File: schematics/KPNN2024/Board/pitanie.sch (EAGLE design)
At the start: 32 parts

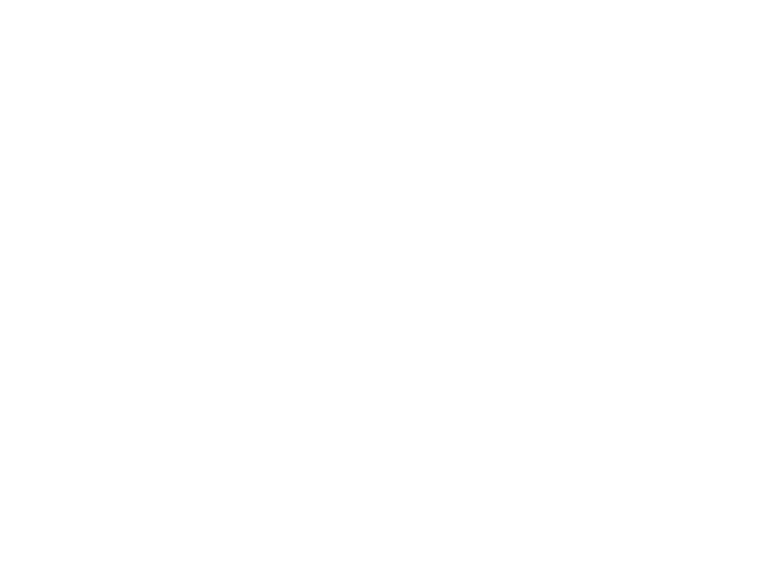
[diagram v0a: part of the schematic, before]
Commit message: я смотрел рика и морти вместо работать
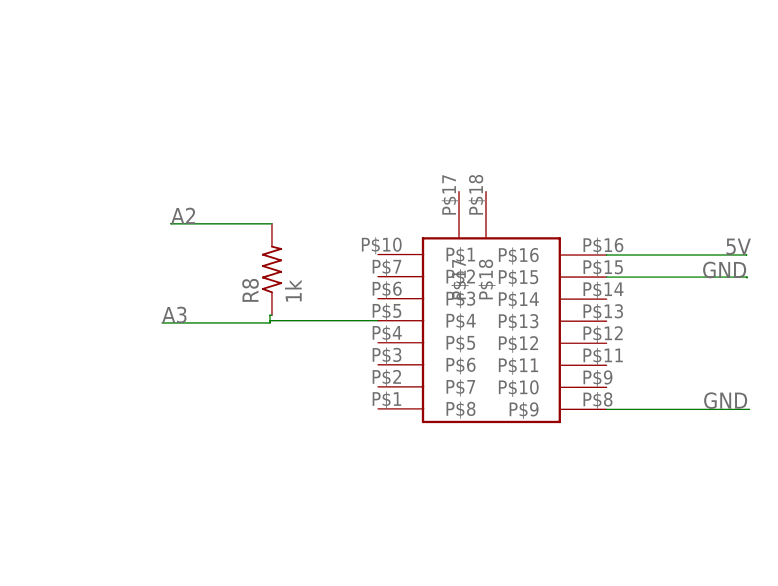
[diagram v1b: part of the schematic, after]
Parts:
- added R8: 1k, rcl:R-US_R0603
- added TMC: DRIVER_TMC2209, UNKNOWN-2024:DRIVER_TMC2209
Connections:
- new net 5V: TMC.P$16
- new net A2: R8.2
- new net A3: R8.1, TMC.P$4
- net GND: now also TMC.P$15, TMC.P$9
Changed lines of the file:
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@@
 <setting verticaltext="up"/>
 </settings>
-<grid distance="0.1" unitdist="inch" unit="inch" style="lines" multiple="1" display="no" altdistance="0.01" altunitdist="inch" altunit="inch"/>
+<grid distance="1" unitdist="mm" unit="mm" style="lines" multiple="1" display="no" altdistance="0.05" altunitdist="mm" altunit="mm"/>
 <layers>
 <layer number="1" name="Top" color="4" fill="1" visible="no" active="no"/>
@@
 <part name="LIS" library="CanCubeSat" deviceset="LIS3MDL-GY" device=""/>
 <part name="R7" library="rcl" library_urn="urn:adsk.eagle:library:334" deviceset="R-US_" device="R0603" package3d_urn="urn:adsk.eagle:package:23555/3" value="2k"/>
+<part name="TMC" library="UNKNOWN-2024" deviceset="DRIVER_TMC2209" device=""/>
+<part name="R8" library="rcl" library_urn="urn:adsk.eagle:library:334" deviceset="R-US_" device="R0603" package3d_urn="urn:adsk.eagle:package:23555/3" value="1k"/>
 </parts>
 <sheets>
@@
 <attribute name="NAME" x="117.8814" y="85.09" size="1.778" layer="95" rot="R90"/>
 <attribute name="VALUE" x="122.682" y="85.09" size="1.778" layer="96" rot="R90"/>
+</instance>
+<instance part="TMC" gate="G$1" x="362" y="78" smashed="yes"/>
+<instance part="R8" gate="G$1" x="345.22" y="94.94" smashed="yes" rot="R90">
+<attribute name="NAME" x="343.7214" y="91.13" size="1.778" layer="95" rot="R90"/>
+<attribute name="VALUE" x="348.522" y="91.13" size="1.778" layer="96" rot="R90"/>
 </instance>
 </instances>
@@
 <label x="213.36" y="121.92" size="1.778" layer="95"/>
 </segment>
+<segment>
+<pinref part="TMC" gate="G$1" pin="P$9"/>
+<wire x1="382.4" y1="79.4" x2="398.244984375" y2="79.4" width="0.1524" layer="91"/>
+<wire x1="398.244984375" y1="79.4" x2="398.244984375" y2="79.3966125" width="0.1524" layer="91"/>
+<label x="393.112159375" y="79.48539375" size="1.778" layer="95"/>
+</segment>
+<segment>
+<pinref part="TMC" gate="G$1" pin="P$15"/>
+<wire x1="382.4" y1="94.1" x2="398" y2="94.1" width="0.1524" layer="91"/>
+<wire x1="398" y1="94.1" x2="398" y2="94" width="0.1524" layer="91"/>
+<label x="393" y="94" size="1.778" layer="95"/>
+</segment>
 </net>
 <net name="8V" class="0">
@@
 </segment>
 </net>
+<net name="A3" class="0">
+<segment>
+<pinref part="TMC" gate="G$1" pin="P$4"/>
+<wire x1="357" y1="89.25" x2="345" y2="89.25" width="0.1524" layer="91"/>
+<wire x1="345" y1="89.25" x2="345" y2="89" width="0.1524" layer="91"/>
+<wire x1="345" y1="89" x2="333" y2="89" width="0.1524" layer="91"/>
+<pinref part="R8" gate="G$1" pin="1"/>
+<wire x1="345" y1="89.25" x2="345" y2="89.86" width="0.1524" layer="91"/>
+<wire x1="345" y1="89.86" x2="345.22" y2="89.86" width="0.1524" layer="91"/>
+<label x="333" y="89" size="1.778" layer="95"/>
+</segment>
+</net>
+<net name="A2" class="0">
+<segment>
+<pinref part="R8" gate="G$1" pin="2"/>
+<wire x1="345.22" y1="100.02" x2="334" y2="100.02" width="0.1524" layer="91"/>
+<wire x1="334" y1="100.02" x2="334" y2="100" width="0.1524" layer="91"/>
+<label x="334" y="100" size="1.778" layer="95"/>
+</segment>
+</net>
+<net name="5V" class="0">
+<segment>
+<pinref part="TMC" gate="G$1" pin="P$16"/>
+<wire x1="382.4" y1="96.55" x2="397.958121875" y2="96.55" width="0.1524" layer="91"/>
+<wire x1="397.958121875" y1="96.55" x2="397.958121875" y2="96.542290625" width="0.1524" layer="91"/>
+<label x="395.55" y="96.6" size="1.778" layer="95"/>
+</segment>
+</net>
